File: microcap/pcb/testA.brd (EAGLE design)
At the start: 99 parts

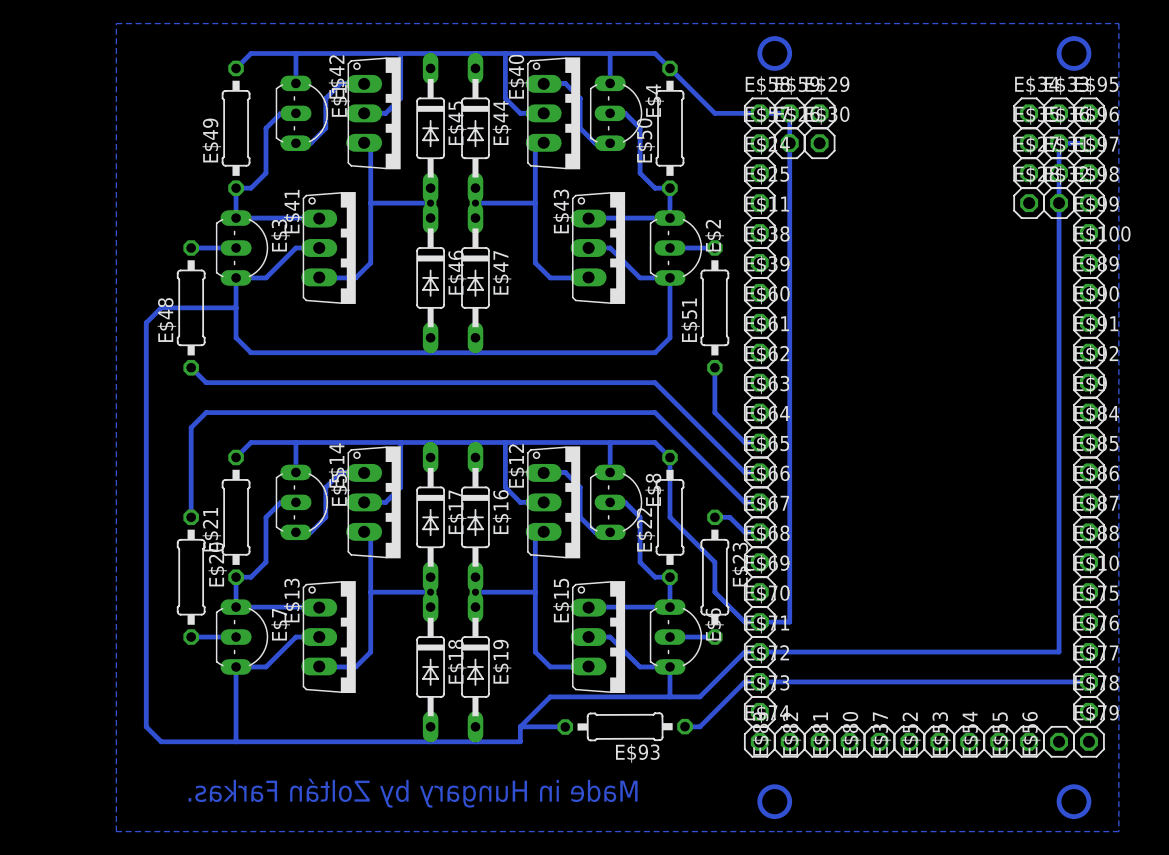
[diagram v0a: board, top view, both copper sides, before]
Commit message: pcb test pdf added
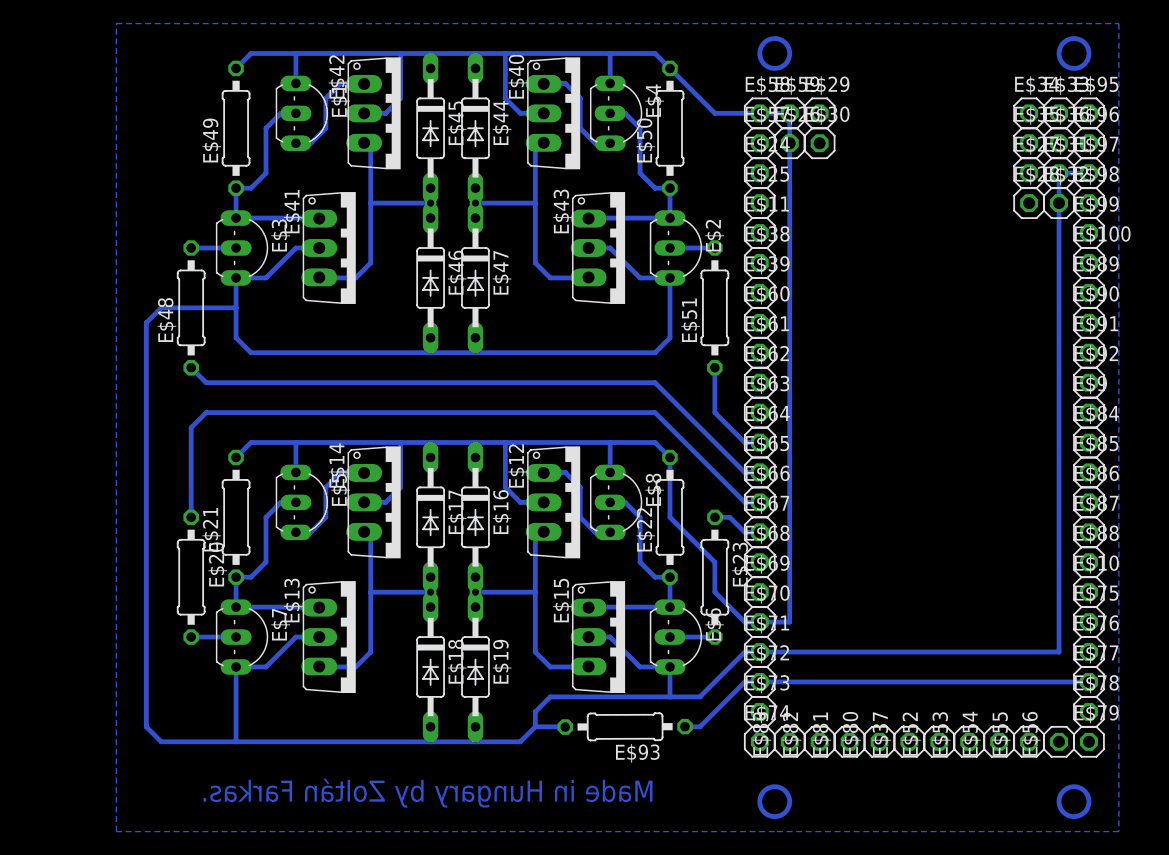
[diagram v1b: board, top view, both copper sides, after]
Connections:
- net S$8: now also E$97.1; no longer E$36.1, E$96.1
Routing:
- net S$8: track 265.5 -> 261.7 mm
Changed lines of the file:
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@@
 <layer number="21" name="tPlace" color="7" fill="1" visible="yes" active="yes"/>
 <layer number="22" name="bPlace" color="7" fill="1" visible="yes" active="yes"/>
-<layer number="23" name="tOrigins" color="15" fill="1" visible="yes" active="yes"/>
-<layer number="24" name="bOrigins" color="15" fill="1" visible="yes" active="yes"/>
+<layer number="23" name="tOrigins" color="15" fill="1" visible="no" active="yes"/>
+<layer number="24" name="bOrigins" color="15" fill="1" visible="no" active="yes"/>
 <layer number="25" name="tNames" color="7" fill="1" visible="no" active="yes"/>
 <layer number="26" name="bNames" color="7" fill="1" visible="no" active="yes"/>
@@
 <circle x="109.22" y="34.29" radius="1.27" width="0.4064" layer="16"/>
 <circle x="83.82" y="34.29" radius="1.27" width="0.4064" layer="16"/>
-<text x="72.39" y="34.29" size="1.778" layer="16" rot="MR0">Made in Hungary by Zoltán Farkas.</text>
+<text x="73.66" y="34.29" size="1.778" layer="16" rot="MR0">Made in Hungary by Zoltán Farkas.</text>
 </plain>
 <attributes>
@@
 <wire x1="38.1" y1="76.2" x2="38.1" y2="73.66" width="0.4064" layer="16"/>
 <wire x1="54.61" y1="72.39" x2="39.37" y2="72.39" width="0.4064" layer="16"/>
-<contactref element="E$96" pad="1"/>
-<contactref element="E$36" pad="1"/>
-<wire x1="110.49" y1="90.17" x2="107.95" y2="90.17" width="0.4064" layer="16"/>
-<wire x1="107.95" y1="90.17" x2="107.95" y2="46.99" width="0.4064" layer="16"/>
 <contactref element="E$71" pad="1"/>
+<wire x1="107.95" y1="87.63" x2="107.95" y2="46.99" width="0.4064" layer="16"/>
 <wire x1="82.55" y1="46.99" x2="81.28" y2="46.99" width="0.4064" layer="16"/>
 <wire x1="82.55" y1="46.99" x2="107.95" y2="46.99" width="0.4064" layer="16"/>
@@
 <wire x1="30.48" y1="74.93" x2="31.75" y2="76.2" width="0.4064" layer="16"/>
 <wire x1="31.75" y1="39.37" x2="30.48" y2="40.64" width="0.4064" layer="16"/>
-<wire x1="62.23" y1="39.37" x2="62.23" y2="40.64" width="0.4064" layer="16"/>
-<wire x1="62.23" y1="40.64" x2="64.77" y2="43.18" width="0.4064" layer="16"/>
+<wire x1="63.5" y1="41.91" x2="64.77" y2="43.18" width="0.4064" layer="16"/>
 <wire x1="64.77" y1="43.18" x2="74.93" y2="43.18" width="0.4064" layer="16"/>
 <wire x1="74.93" y1="43.18" x2="77.47" y2="43.18" width="0.4064" layer="16"/>
-<wire x1="66.04" y1="40.64" x2="62.23" y2="40.64" width="0.4064" layer="16"/>
+<contactref element="E$97" pad="1"/>
+<wire x1="110.49" y1="87.63" x2="107.95" y2="87.63" width="0.4064" layer="16"/>
+<wire x1="63.5" y1="41.91" x2="63.5" y2="40.64" width="0.4064" layer="16"/>
+<wire x1="66.04" y1="40.64" x2="63.5" y2="40.64" width="0.4064" layer="16"/>
+<wire x1="63.5" y1="40.64" x2="62.23" y2="39.37" width="0.4064" layer="16"/>
 </signal>
 <signal name="S$1">
